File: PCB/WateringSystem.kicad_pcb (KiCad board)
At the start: 2 copper layers, 99.6 x 72.1 mm, 48 parts, among them J1 Jack-DC, J2 Conn_01x02, J3 Conn_01x02, J4 Conn_01x04, J5 Conn_01x04, J6 Conn_01x04, J7 Conn_01x04, Q1 Q_NMOS_GDS, Q2 Q_NMOS_GDS, Q3 Q_NMOS_GDS, Q4 Q_NMOS_GDS, SW1 Rotary_Encoder_Switch, SW2 SW_Push, SW3 SW_Push, SW4 SW_Push, SW5 SW_Push, U1 arduino_mini

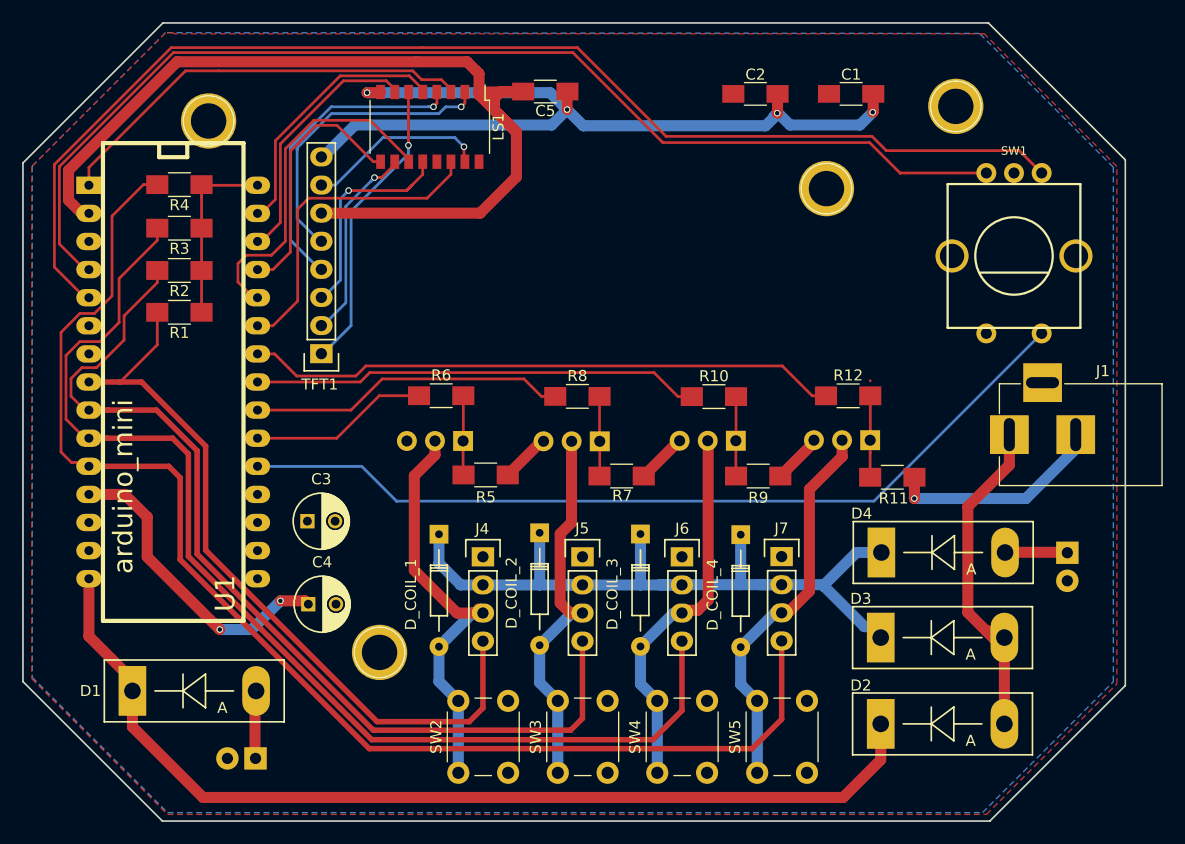
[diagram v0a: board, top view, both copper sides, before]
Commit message: fixed and updated PCB
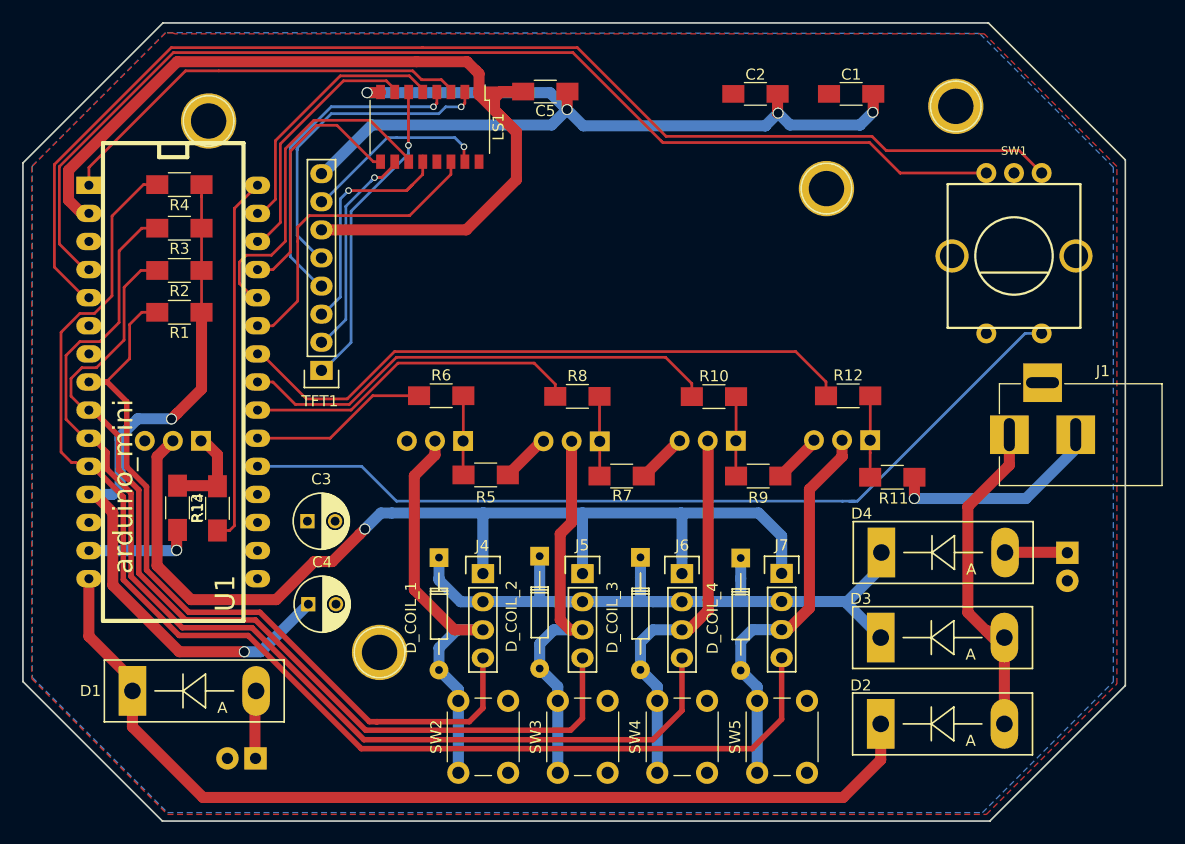
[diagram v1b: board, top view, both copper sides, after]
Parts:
- added Q5: Q_NMOS_GDS, TO_SOT_Packages_THT:TO-220_Vertical, B.Cu at (63.3, 113.5)
- added R13: 1k, Resistors_SMD:R_1206_HandSoldering, F.Cu at (64.8, 119.6)
- added R14: 10k, Resistors_SMD:R_1206_HandSoldering, F.Cu at (61.2, 119.6)
- moved D_COIL_1 2.11 mm to (84.8, 124.1)
- moved D_COIL_2 2.11 mm to (93.9, 123.9)
- moved D_COIL_3 2.11 mm to (103.1, 124.0)
- moved D_COIL_4 2.11 mm to (112.1, 124.1)
- moved J4 1.52 mm to (88.8, 125.5)
- moved J5 1.52 mm to (97.8, 125.5)
- moved J6 1.52 mm to (106.8, 125.5)
- moved J7 1.52 mm to (115.8, 125.5)
- moved TFT1 1.51 mm to (74.2, 107.2)
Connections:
- J4 pad 1: GND -> Net-(J4-Pad1)
- J5 pad 1: GND -> Net-(J4-Pad1)
- J6 pad 1: GND -> Net-(J4-Pad1)
- J7 pad 1: GND -> Net-(J4-Pad1)
- R1 pad 1: Net-(R1-Pad1) -> +5V
- R2 pad 1: Net-(R1-Pad1) -> +5V
- R3 pad 1: Net-(R1-Pad1) -> +5V
- R4 pad 1: Net-(R1-Pad1) -> +5V
- U1 pad 30: Net-(R1-Pad1) -> Net-(R13-Pad1)
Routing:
- net Net-(J4-Pad1): track 0.00 -> 93.6 mm, vias 0 -> 1
- net +5V: track 28.2 -> 67.1 mm
- net Net-(R13-Pad1): track 0.00 -> 33.2 mm
- net Net-(R1-Pad1): track 16.6 -> 0.00 mm
- net GND: track 112.0 -> 122.4 mm, vias 5 -> 6
- net Net-(Q5-Pad1): track 0.00 -> 8.49 mm
- net Net-(D3-Pad1): track 72.7 -> 67.3 mm
- net Net-(R10-Pad1): track 40.5 -> 44.0 mm
- net Net-(R12-Pad1): track 54.1 -> 57.2 mm
- net Net-(J4-Pad4): track 68.4 -> 70.6 mm
- net Net-(J7-Pad4): track 118.5 -> 116.6 mm
- net Net-(R8-Pad1): track 28.7 -> 30.6 mm
- net Net-(LS1-Pad4): track 28.6 -> 29.9 mm
- net Net-(LS1-Pad2): track 27.5 -> 28.9 mm
- net Net-(LS1-Pad6): track 27.2 -> 28.5 mm
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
